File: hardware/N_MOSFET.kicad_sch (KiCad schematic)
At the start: 4 parts, among them Q4 Q_NMOS_DGS

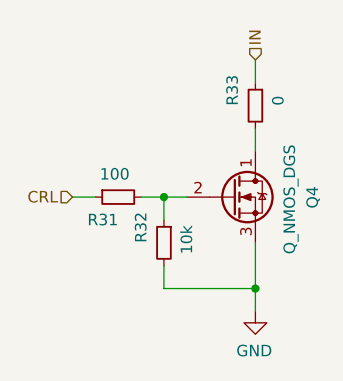
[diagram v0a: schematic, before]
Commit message: minor improvements
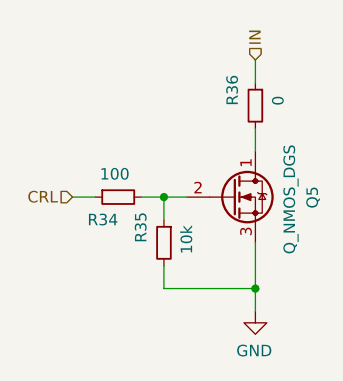
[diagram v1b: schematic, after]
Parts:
- renumbered Q4 to Q5, R31 to R34, R32 to R35, R33 to R36
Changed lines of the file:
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@@
   (symbol (lib_id "Device:Q_NMOS_DGS") (at 161.29 102.87 0)
     (in_bom yes) (on_board yes)
-    (property "Reference" "Q4" (id 0) (at 170.18 104.14 90)
+    (property "Reference" "Q5" (id 0) (at 170.18 104.14 90)
       (effects (font (size 1.27 1.27)) (justify left))
     )
@@
   (symbol (lib_id "Device:R_Small") (at 153.67 107.95 0) (mirror y)
     (in_bom yes) (on_board yes)
-    (property "Reference" "R32" (id 0) (at 151.13 107.95 90)
+    (property "Reference" "R35" (id 0) (at 151.13 107.95 90)
       (effects (font (size 1.27 1.27)) (justify left))
     )
@@
   (symbol (lib_id "Device:R_Small") (at 148.59 102.87 90) (mirror x)
     (in_bom yes) (on_board yes)
-    (property "Reference" "R31" (id 0) (at 148.59 105.41 90)
+    (property "Reference" "R34" (id 0) (at 148.59 105.41 90)
       (effects (font (size 1.27 1.27)) (justify left))
     )
@@
   (symbol (lib_id "Device:R_Small") (at 163.83 92.71 0) (mirror y)
     (in_bom yes) (on_board yes)
-    (property "Reference" "R33" (id 0) (at 161.29 92.71 90)
+    (property "Reference" "R36" (id 0) (at 161.29 92.71 90)
       (effects (font (size 1.27 1.27)) (justify left))
     )
